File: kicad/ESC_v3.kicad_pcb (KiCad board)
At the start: 4 copper layers, 50 x 50 mm, 175 parts, among them J1 Conn_01x05_Pin, J2 Conn_01x05_Pin, J3 Conn_01x01_Pin, J4 Conn_01x06_Pin, J5 Conn_01x02_Pin, J6 Conn_01x06_Pin, J7 Conn_01x02_Pin, J8 Conn_01x04_Pin, J9 Conn_01x02_Pin, Q1 RH6L040BGTB1, Q10 RH6L040BGTB1, Q11 RH6L040BGTB1, Q12 RH6L040BGTB1, Q2 RH6L040BGTB1, Q3 RH6L040BGTB1, Q4 RH6L040BGTB1, Q5 RH6L040BGTB1, Q6 RH6L040BGTB1, Q7 RH6L040BGTB1, Q8 RH6L040BGTB1, Q9 RH6L040BGTB1, SW2 SW_Nidec_CAS-120A1, U1 L6387, U10 BD4104, U11 AMS1117-5.0, U12 ACS711xEXLT-15AB, U13 LM2937xMP, U14 MCP9700x-ETT, U15 MAX40200AUK, U19 STM32G431CBUx, U2 L6387, U3 L6387, U4 L6387, U5 L6387, U6 L6387, U7 AMS1117-3.3, U8 ACS711xEXLT-15AB, U9 ACS711xEXLT-15AB

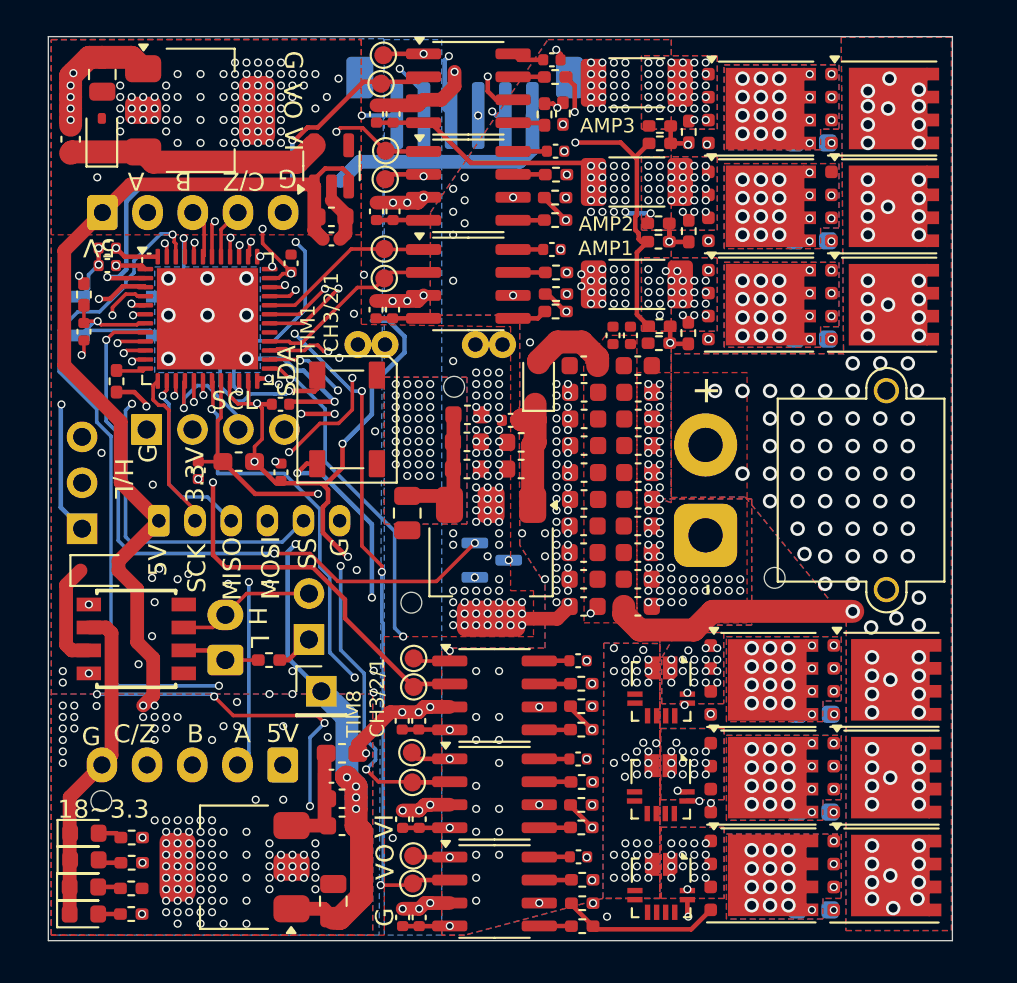
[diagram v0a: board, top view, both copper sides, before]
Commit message: test
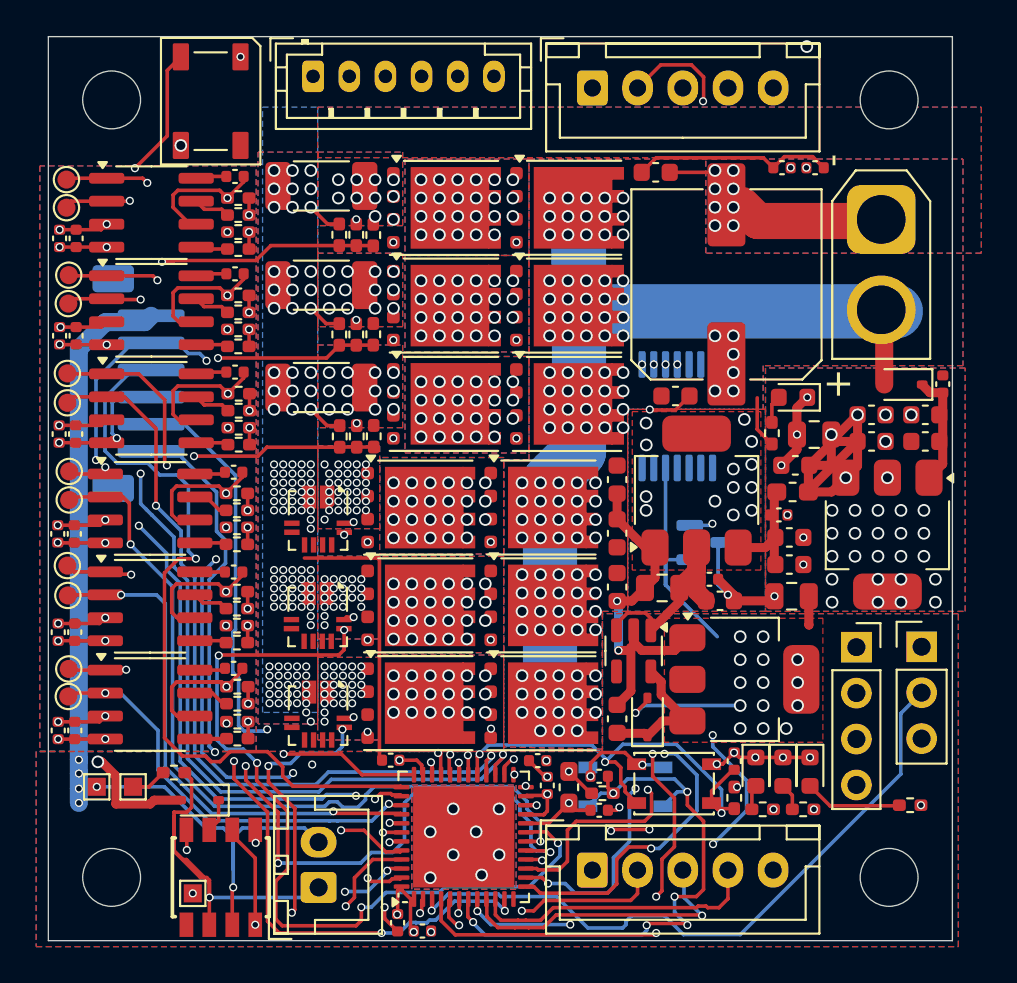
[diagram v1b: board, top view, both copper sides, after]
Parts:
- removed BZ1: Buzzer, jisaku:buzzer_unified
- removed C31, C45, C46, C47, C48, C49, C50, C51, C52, C53, C54, C55, C56, C57: 22uF, Capacitor_SMD:C_0603_1608Metric
- removed J3: Conn_01x01_Pin, Connector_PinHeader_2.54mm:PinHeader_1x01_P2.54mm_Vertical
- removed J5: Conn_01x02_Pin, Connector_PinHeader_2.54mm:PinHeader_1x02_P2.54mm_Vertical
- removed R29: 100, Resistor_SMD:R_0402_1005Metric_Pad0.72x0.64mm_HandSolder
- removed REF** (x4): ToolingHole_1.152mm, MountingHole:ToolingHole_1.152mm
- added C39: 0.1u, Capacitor_SMD:C_0402_1005Metric, F.Cu at (87.9, 90.1)
- added H1: MountingHole, MountingHole:MountingHole_3.2mm_M3, F.Cu at (53.5, 53.5)
- added H2: MountingHole, MountingHole:MountingHole_3.2mm_M3, F.Cu at (53.5, 96.5)
- added H3: MountingHole, MountingHole:MountingHole_3.2mm_M3, F.Cu at (96.5, 53.5)
- added H4: MountingHole, MountingHole:MountingHole_3.2mm_M3, F.Cu at (96.5, 96.5)
- added R5: 10k, Resistor_SMD:R_0402_1005Metric_Pad0.72x0.64mm_HandSolder, F.Cu at (87.9, 92.1)
- added TP13: TestPoint, TestPoint:TestPoint_Pad_1.0x1.0mm, F.Cu at (54.7, 91.5)
- added TP14: TestPoint, TestPoint:TestPoint_Pad_1.0x1.0mm, F.Cu at (52.7, 91.5)
- added TP15: TestPoint, TestPoint:TestPoint_Pad_1.0x1.0mm, F.Cu at (58.0, 97.4)
- added U16: AS5048A, Package_SO:TSSOP-14_4.4x5mm_P0.65mm, B.Cu at (84.8, 71.0)
- added button1: SW_Push, Button_Switch_SMD:SW_SPST_PTS810, F.Cu at (84.6, 91.3)
- C24: value 22uF -> 470u; footprint Capacitor_SMD:C_0603_1608Metric -> Capacitor_SMD:C_Elec_10x10.2
- J1, J2: footprint Connector_JST:JST_XH_S5B-XH-A_1x05_P2.50mm_Horizontal -> Connector_JST:JST_XH_B5B-XH-A_1x05_P2.50mm_Vertical; moved to F.Cu
- J4, J8, SW2: moved to F.Cu
- J7: footprint Connector_JST:JST_XH_S2B-XH-A_1x02_P2.50mm_Horizontal -> Connector_JST:JST_XH_B2B-XH-A_1x02_P2.50mm_Vertical; moved to F.Cu
- J9: footprint Connector_AMASS:AMASS_XT30PW-M_1x02_P2.50mm_Horizontal -> Connector_AMASS:AMASS_XT30U-M_1x02_P5.0mm_Vertical
- R10, R14, R18, R22, R26, R4: footprint Resistor_SMD:R_0603_1608Metric_Pad0.98x0.95mm_HandSolder -> Resistor_SMD:R_0402_1005Metric_Pad0.72x0.64mm_HandSolder; moved to F.Cu
- moved G*** 48.2 mm to (125.6, 94.1)
- moved G*** 48.2 mm to (120.5, 90.3)
- moved G*** 48.2 mm to (119.9, 96.5)
- moved G*** 48.2 mm to (117.1, 90.4)
- moved C30 47.8 mm to (91.1, 80.9), turned to 180 degrees
- moved SW2 46.9 mm to (98.3, 83.7)
- moved D13 46.0 mm to (91.2, 70.0), turned to 180 degrees
- moved C29 44.1 mm to (81.5, 87.7)
- moved D3 44.0 mm to (83.1, 87.6)
- moved U7 43.5 mm to (88.5, 85.5)
- moved R59 43.5 mm to (97.7, 92.5)
- moved R56 41.9 mm to (90.0, 71.9), turned to -90 degrees
- moved J8 41.1 mm to (94.7, 83.8), turned to 0 degrees
- moved D17 40.9 mm to (92.1, 90.7), turned to -90 degrees
- moved C37 40.6 mm to (69.3, 99.0), turned to -90 degrees
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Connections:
- R48 pad 1: +3.3V -> VREF
- R49 pad 1: +3.3V -> VREF
- R54 pad 1: +3.3V -> VREF
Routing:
- net GND: track 228.4 -> 108.5 mm, vias 340 -> 194
- net +5V: track 75.3 -> 177.9 mm, vias 104 -> 17
- net +3.3V: track 152.6 -> 63.6 mm, vias 94 -> 28
- net +12V: track 56.0 -> 139.7 mm, vias 53 -> 14
- net EXTI13: track 2.83 -> 62.1 mm, vias 0 -> 1
- net SPI1_SCK: track 8.97 -> 68.2 mm, vias 0 -> 3
- net SS: track 26.3 -> 85.2 mm, vias 2 -> 4
- net TIM3_CH1: track 7.64 -> 65.2 mm, vias 1 -> 4
- net TIM3_CH2: track 2.73 -> 59.0 mm, vias 0 -> 1
- net SPI1_MISO: track 10.2 -> 64.4 mm, vias 1 -> 3
- net SPI1_MOSI: track 12.1 -> 62.2 mm, vias 1 -> 2
- net TIM4_CH2: track 16.9 -> 63.3 mm
- net ADC2_IN10: track 66.5 -> 25.1 mm, vias 8 -> 4
- net TIM1_CH1: track 23.2 -> 58.9 mm
- net TIM1_CH3: track 9.81 -> 44.9 mm, vias 0 -> 2
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- added copper zone on In3.Cu, net +12V
- added copper zone on In3.Cu, net +3.3V
- added copper zone on In3.Cu, net +5V
- added copper zone on In3.Cu, net /POWER/halfHbridge4/GND_mech
- added copper zone on In4.Cu, net /POWER/halfHbridge4/GND_mech
- added copper zone on In3.Cu, net /POWER/halfHbridge4/out1
- added copper zone on In4.Cu, net /POWER/halfHbridge4/out1
- added copper zone on In3.Cu, net /POWER/halfHbridge5/GND_mech
- added copper zone on In4.Cu, net /POWER/halfHbridge5/GND_mech
- added copper zone on In3.Cu, net /POWER/halfHbridge5/out1
- added copper zone on In4.Cu, net /POWER/halfHbridge5/out1
- added copper zone on In3.Cu, net /POWER/halfHbridge6/GND_mech
- added copper zone on In4.Cu, net /POWER/halfHbridge6/GND_mech
- added copper zone on In3.Cu, net /POWER/halfHbridge6/out1
- added copper zone on In4.Cu, net /POWER/halfHbridge6/out1
- added copper zone on In3.Cu, net /POWER/halfHbridge7/GND_mech
- added copper zone on In4.Cu, net /POWER/halfHbridge7/GND_mech
- added copper zone on In3.Cu, net /POWER/halfHbridge7/out1
- added copper zone on In4.Cu, net /POWER/halfHbridge7/out1
- added copper zone on In3.Cu, net /POWER/halfHbridge8/GND_mech
- added copper zone on In4.Cu, net /POWER/halfHbridge8/GND_mech
- added copper zone on In3.Cu, net /POWER/halfHbridge8/out1
- added copper zone on In4.Cu, net /POWER/halfHbridge8/out1
- added copper zone on In3.Cu, net /POWER/halfHbridge9/GND_mech
- added copper zone on In4.Cu, net /POWER/halfHbridge9/GND_mech
- added copper zone on In3.Cu, net /POWER/halfHbridge9/out1
- added copper zone on In4.Cu, net /POWER/halfHbridge9/out1
- added copper zone on In3.Cu, net GND
- added copper zone on In4.Cu, net GND
- added copper zone on In3.Cu, net VCC
- added copper zone on In4.Cu, net VCC
- removed copper zone on In1.Cu, net +12V
- removed copper zone on In1.Cu, net +3.3V
- removed copper zone on In1.Cu, net +5V
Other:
- copper layers 4 -> 6
- board text removed: "18~3.3"
- board text removed: "3.3V"
- board text removed: "5V"
- board text removed: "A"
- board text removed: "AMP1"
- board text removed: "AMP2"
- board text removed: "AMP3"
- board text removed: "B"
- board text removed: "C/Z"
- board text removed: "CLK"
- board text removed: "DIO"
- board text removed: "G"
- board text removed: "GND"
- board text removed: "H"
- board text removed: "H/L"
- board text removed: "L"
- board text removed: "L/H"
- board text removed: "MISO"
- board text removed: "MOSI"
- board text removed: "NRST"
- board text removed: "RX"
- board text removed: "SCK"
- board text removed: "SCL"
- board text removed: "SDA"
- board text removed: "SS"
- board text removed: "TIM1 CH3/2/1"
- board text removed: "TIM8 CH3/2/1"
- board text removed: "TX"
- board text removed: "VI"
- board text removed: "VO"
